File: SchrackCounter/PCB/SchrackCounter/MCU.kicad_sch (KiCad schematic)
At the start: 0 parts

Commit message: update
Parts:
- added C?: 100nF.mcu, Capacitor_SMD:C_0805_2012Metric_Pad1.18x1.45mm_HandSolder, symbol Device:C
- added C?: 10uF.mcu, Capacitor_Tantalum_SMD:CP_EIA-3216-18_Kemet-A_Pad1.58x1.35mm_HandSolder, symbol Device:C_Polarized
- added U?: ESP32-S3-WROOM-1, PCM_Espressif:ESP32-S3-WROOM-1, symbol sumec_sch_lib:ESP32-S3-WROOM-1_CUSTOM_made_by_bismarx
- added U?: ESP32-S3-WROOM-2, PCM_Espressif:ESP32-S3-WROOM-2, symbol PCM_Espressif:ESP32-S3-WROOM-2
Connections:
- new net: U?.1 (GND), U?.40 (GND), U?.41 (GND)
- new net +3V3: C?.1, C?.1, U?.2 (3V3)
- new net BOOT: U?.27 (IO0)
- new net D+: U?.14 (IO20)
- new net D-: U?.13 (IO19)
- new net EN: U?.3 (EN)
- new net GND: C?.2, C?.2, U?.1 (GND), U?.40 (GND), U?.41 (GND)
- new net IN1: U?.33 (IO40)
- new net IN2: U?.34 (IO41)
- new net IPROPI_ADC: U?.29 (IO36)
- new net IR MODULE: U?.28 (IO35)
- new net LED1: U?.23 (IO21)
- new net LED2: U?.22 (IO14)
- new net LED3: U?.21 (IO13)
- new net OUT 1A: U?.18 (IO10)
- new net OUT 1B: U?.17 (IO9)
- new net OUT 2A: U?.19 (IO11)
- new net OUT 2B: U?.20 (IO12)
- new net POL 1: U?.5 (IO5)
- new net POL 2: U?.8 (IO15)
- new net POL 3: U?.9 (IO16)
- new net PWM1: U?.35 (IO42)
- new net PWM2: U?.32 (IO39)
- new net QRE1113 A: U?.6 (IO6)
- new net QRE1113 B: U?.7 (IO7)
- new net QRE1113 C: U?.38 (IO2)
- new net RX: U?.36 (RXD0)
- new net SCL: U?.11 (IO18)
- new net SDA: U?.10 (IO17)
- new net SHARP 1: U?.12 (IO8)
- new net SHARP 2: U?.4 (IO4)
- new net TEST PROGRAM 1: U?.25 (IO48)
- new net TEST PROGRAM 2: U?.24 (IO47)
- new net TX: U?.37 (TXD0)
- new net nFAULT: U?.30 (IO37)
- new net nSLEEP: U?.31 (IO38)
- no-connect marks 0 -> 3
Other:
- note added: "Default Configuration of Strapping Pins Strapping Pin Default Configuration Bit Value GPIO0 Pull-up 1 GPIO3 Floating - GPIO45 Pull-down 0 GPIO46 Pull-down 0"
- note added: "ESP32-S3 Datasheet"
- note added: "ESP32-S3-WROOM1-N4"
- note added: "GPIO0 has an internal pullup resistor, so if it is left unconnected then it will pull high."
- note added: "GPIO0, GPIO45, and GPIO46 are connected to the chip's internal weak pull-up/pull-down resistors at chip reset. These resistors determine the default bit values of the strapping pins. Also, these resistors determine the bit values if the strapping pins are connected to an external high-impedance circuit."
- note added: "TEST!!!"
- note added: "Typically these can be used, but you need to make sure they are not in the wrong state during boot. gpio.0 Boot Mode. Weak pullup during reset. (Boot Mode 0=Boot from Flash, 1=Download) gpio.3 JTAG Mode. Weak pull down during reset. (JTAG Config) gpio.45 SPI voltage. Weak pull down during reset. (SPI Voltage 0=3.3v 1=1.8v) gpio.46 Boot mode. Weak pull down during reset. (Enabling/Disabling ROM Me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"
- note added: "working voltage for pins 47 and 48 is 1.8 (test it) Check pins with datasheet, ADC, SP, USB etc Check encoder connection UART connection?"

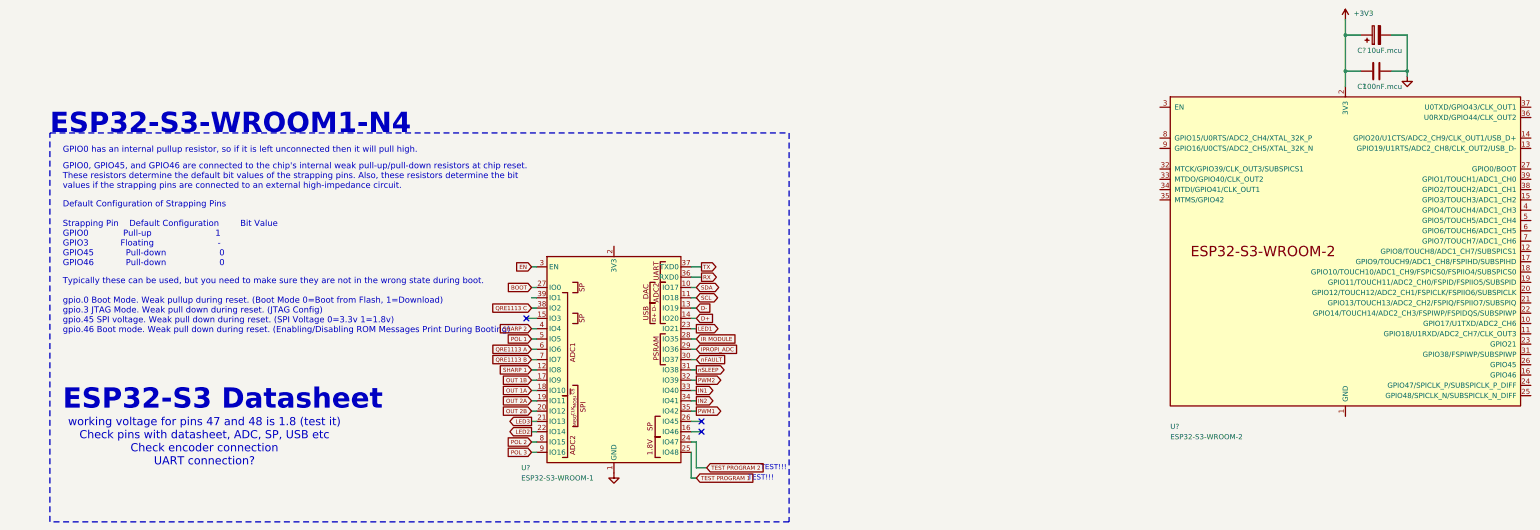
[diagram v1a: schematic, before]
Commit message: Schematic update
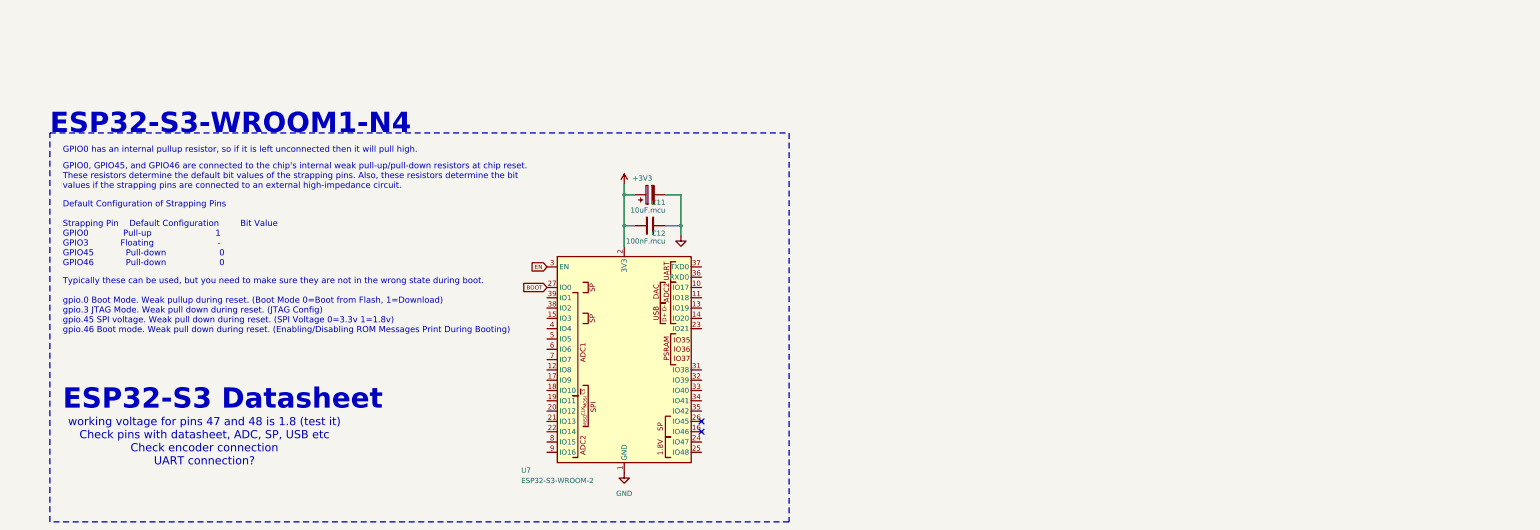
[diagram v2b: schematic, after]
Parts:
- removed U?: ESP32-S3-WROOM-1, PCM_Espressif:ESP32-S3-WROOM-1, symbol sumec_sch_lib:ESP32-S3-WROOM-1_CUSTOM_made_by_bismarx
- removed U?: ESP32-S3-WROOM-2, PCM_Espressif:ESP32-S3-WROOM-2, symbol PCM_Espressif:ESP32-S3-WROOM-2
- added U7: ESP32-S3-WROOM-2, PCM_Espressif:ESP32-S3-WROOM-2, symbol sumec_sch_lib:ESP32-S3-WROOM-2_CUSTOM_made_by_bismarx
- gave numbers to parts that had none: 2
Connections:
- net +3V3: now also U7.2 (3V3)
- net BOOT: now also U7.27 (IO0)
- net EN: now also U7.3 (EN)
- net GND: now also U7.1 (GND), U7.40 (GND), U7.41 (GND)
- no-connect marks 3 -> 2
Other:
- note removed: "TEST!!!"
- moved on the sheet: C11, C12
